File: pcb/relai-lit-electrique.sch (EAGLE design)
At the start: 24 parts, among them K1 DSP1.1A, Q3 2N5484, Q4 2N5484, X1 DSP-3, X2 DSP-3

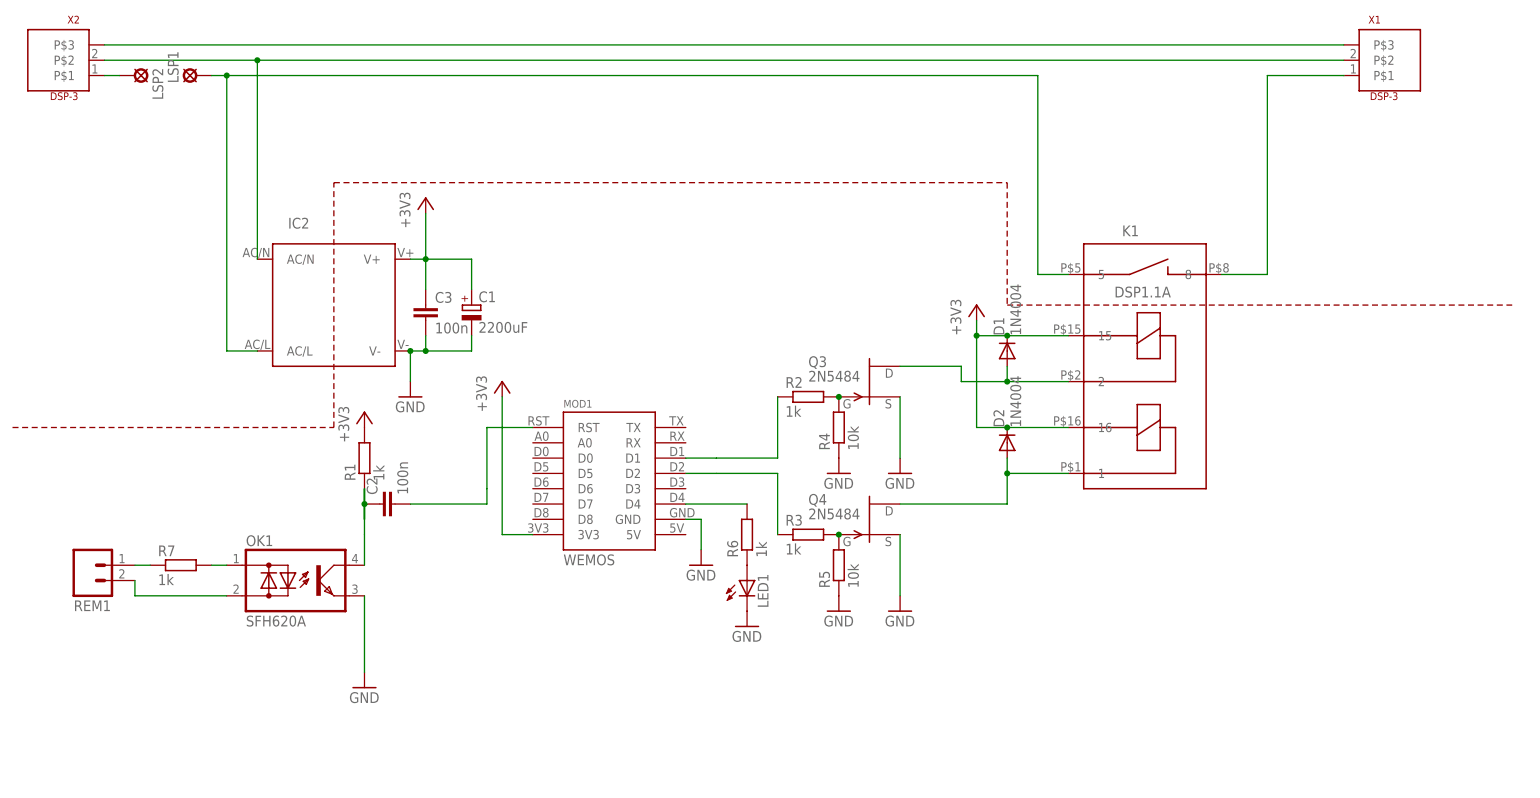
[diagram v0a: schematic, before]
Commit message: update
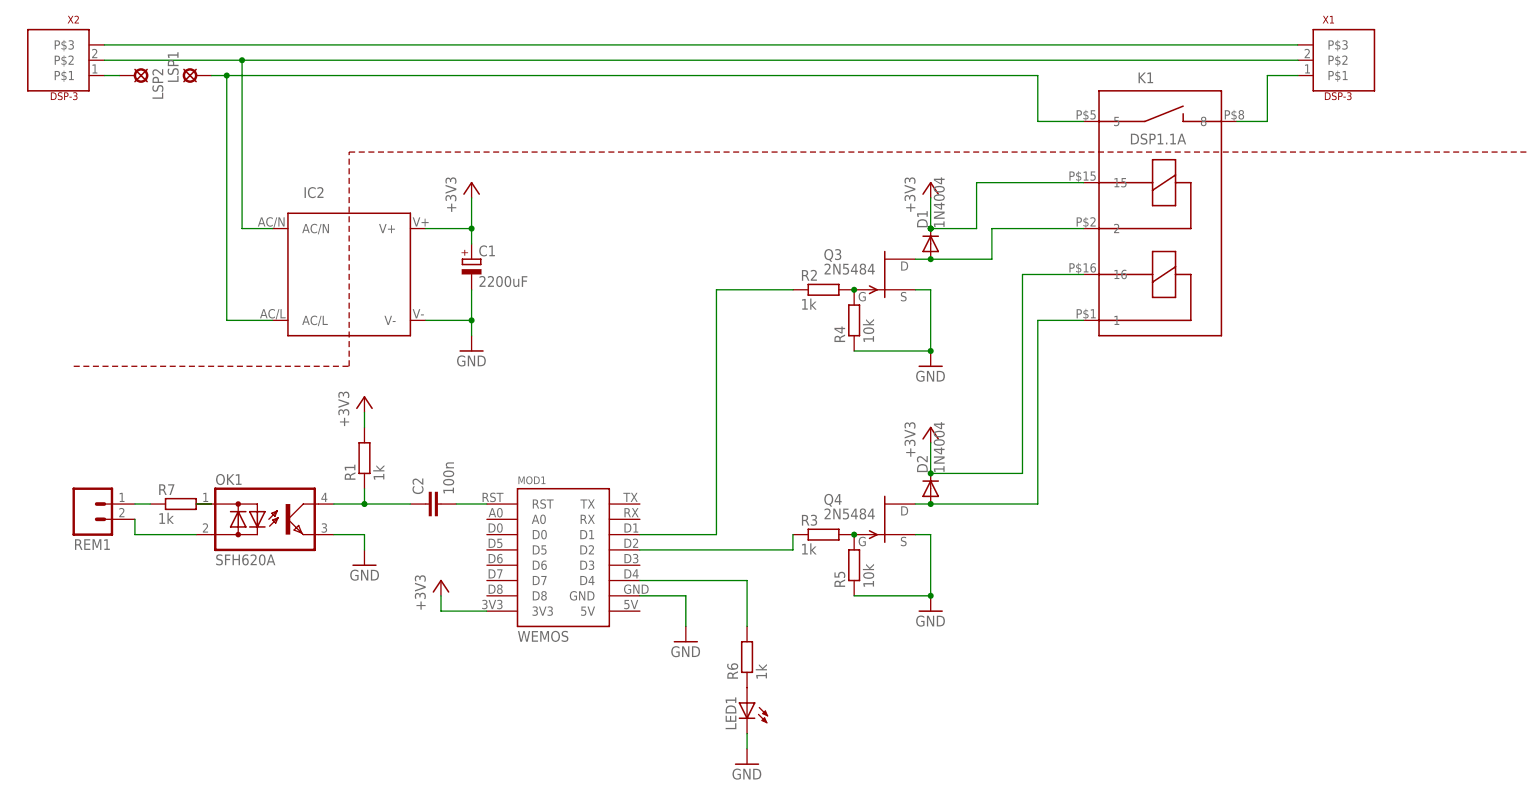
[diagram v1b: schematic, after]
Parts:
- removed C3: 100n, rcl:C-EU025-024X044
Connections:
- net +3V3: no longer C3.1
- net GND: no longer C3.2
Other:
- moved on the sheet: C1, C2, D1, D2, IC2, K1, LED1, MOD1, OK1, Q3, Q4, R2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
